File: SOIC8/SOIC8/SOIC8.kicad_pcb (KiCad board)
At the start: 2 copper layers, 10.7 x 10.7 mm, 5 parts, among them J1 Conn_01x04, J2 Conn_01x04

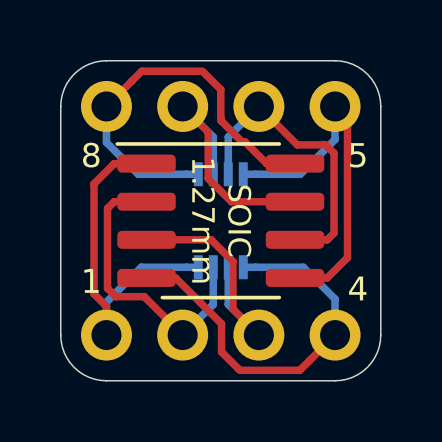
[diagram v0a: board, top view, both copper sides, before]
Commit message: Board Updates
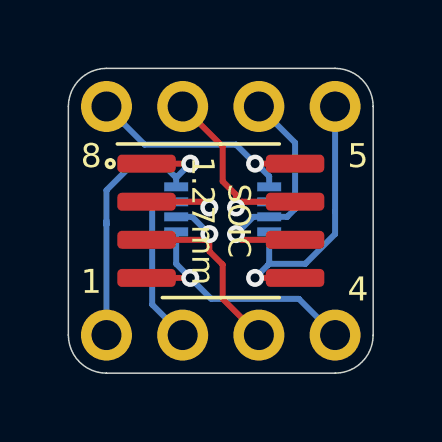
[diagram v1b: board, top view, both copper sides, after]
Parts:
- removed REF**: VSSOP-8_2.3x2mm_P0.5mm, Package_SO:VSSOP-8_2.3x2mm_P0.5mm
- removed SOIC/SOIJ: ATtiny85-20SU, Package_SO:SOIC-8_3.9x4.9mm_P1.27mm
- added J3: SOIC8, Package_SO:SOIC-8_3.9x4.9mm_P1.27mm, F.Cu at (65.0, 33.0)
- added J4: VSSOP8, Package_SO:VSSOP-8_2.3x2mm_P0.5mm, B.Cu at (65.1, 32.6)
- moved G*** 3.45 mm to (65.0, 34.9), turned to 0 degrees
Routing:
- net Net-(J1-Pad1): track 13.4 -> 8.07 mm, vias 0 -> 1
- net Net-(J2-Pad4): track 13.3 -> 8.80 mm, vias 0 -> 1
- net Net-(J1-Pad4): track 11.8 -> 9.92 mm, vias 0 -> 1
- net Net-(J2-Pad1): track 11.8 -> 10.3 mm, vias 0 -> 1
- net Net-(J1-Pad3): track 9.79 -> 8.28 mm, vias 0 -> 1
- net Net-(J1-Pad2): track 8.75 -> 7.33 mm, vias 0 -> 1
- net Net-(J2-Pad3): track 8.77 -> 7.57 mm, vias 0 -> 1
- net Net-(J2-Pad2): track 9.79 -> 8.90 mm, vias 0 -> 1
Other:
- board size 10.7 x 10.7 mm -> 10.2 x 10.2 mm
- net class Default: clearance 0.2 -> 0.127; trace_width 0.25 -> 0.127; via_dia 0.8 -> 0.6; via_drill 0.4 -> 0.3
- rule trace_clearance: 0.2 -> 0.127
- rule trace_min: 0.2 -> 0.127
- board text added: "P=0.5mm"
- board text removed: "VSSOP 0.5mm"
